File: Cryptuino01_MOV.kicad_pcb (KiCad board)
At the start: 2 copper layers, 37.9 x 31.2 mm, 31 parts, among them J1 USB_C_Receptacle_USB2.0, J2 Conn_01x06_Female, J3 Conn_01x08_Female, U1 FT245RL, U2 74HC02, U3 74HC00, U4 ATtiny4313-MU

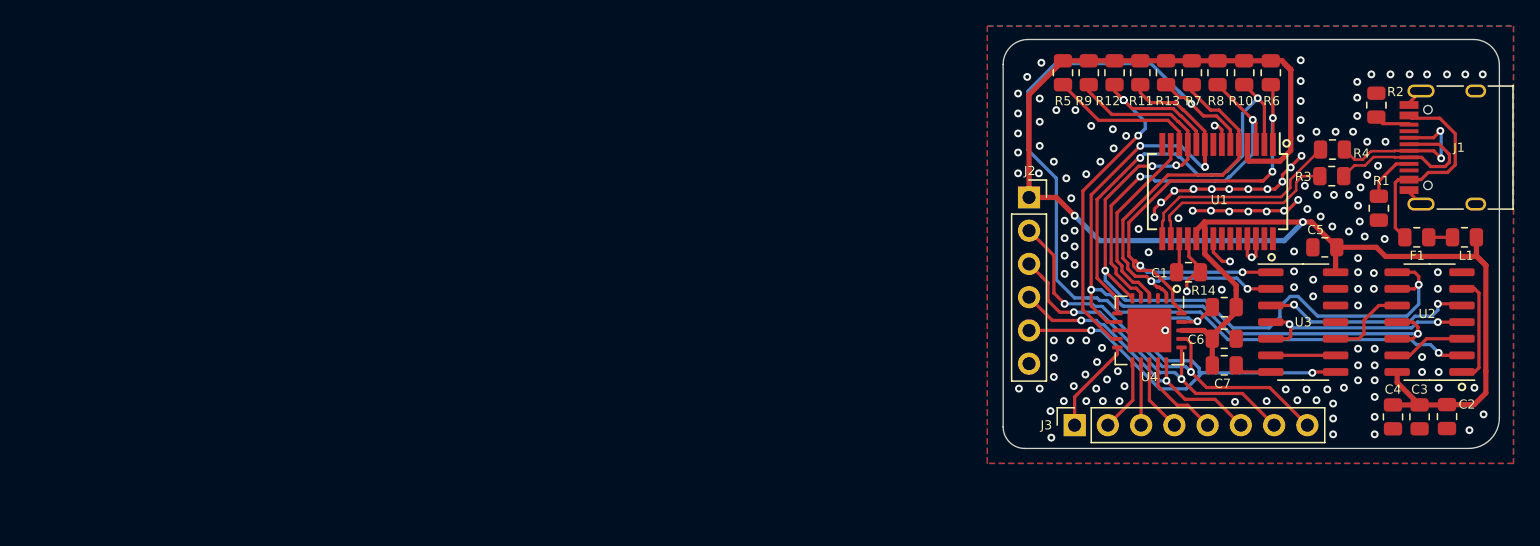
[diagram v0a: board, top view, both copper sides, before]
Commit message: done_nice_now
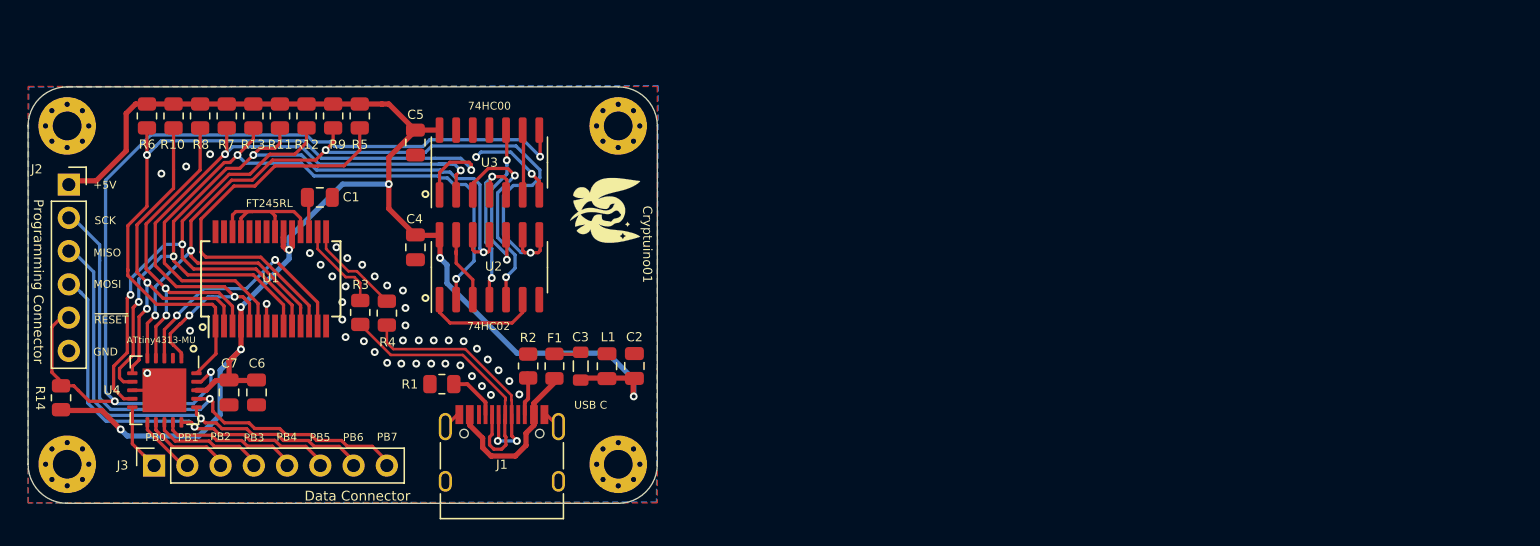
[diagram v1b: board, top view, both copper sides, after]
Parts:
- added G***: LOGO, FairyLogo:fairy_mask, F.Cu at (127.9, 67.2)
- added G***: LOGO, FairyLogo:fairy_silks, F.Cu at (128.0, 64.5)
- added REF**: KiCad-Logo2_6mm_SilkScreen, Symbol:KiCad-Logo2_6mm_SilkScreen, B.Cu at (103.6, 69.8)
- added REF**: MountingHole_2.2mm_M2_Pad_Via, MountingHole:MountingHole_2.2mm_M2_Pad_Via, F.Cu at (129.0, 58.0)
- added REF**: MountingHole_2.2mm_M2_Pad_Via, MountingHole:MountingHole_2.2mm_M2_Pad_Via, F.Cu at (86.9, 58.0)
- added REF**: MountingHole_2.2mm_M2_Pad_Via, MountingHole:MountingHole_2.2mm_M2_Pad_Via, F.Cu at (86.9, 83.9)
- added REF**: MountingHole_2.2mm_M2_Pad_Via, MountingHole:MountingHole_2.2mm_M2_Pad_Via, F.Cu at (129.0, 83.9)
- C1, C2, C3, C4, C5, C6, C7: footprint Resistor_SMD:R_0805_2012Metric -> Capacitor_SMD:C_0805_2012Metric
- F1: footprint Resistor_SMD:R_0805_2012Metric -> Fuse:Fuse_0805_2012Metric
- L1: footprint Resistor_SMD:R_0805_2012Metric -> Inductor_SMD:L_0805_2012Metric
- moved R14 89.1 mm to (86.4, 78.8), turned to 270 degrees
- moved R6 85.9 mm to (93.0, 57.3)
- moved R10 81.9 mm to (95.0, 57.3)
- moved R8 77.8 mm to (97.0, 57.3)
- moved J1 77.3 mm to (120.1, 84.1), turned to 0 degrees
- moved C7 76.1 mm to (99.2, 78.4), turned to 270 degrees
- moved C4 75.8 mm to (113.5, 67.3)
- moved U4 75.4 mm to (94.3, 78.2)
- moved R3 74.9 mm to (109.3, 72.3), turned to 270 degrees
- moved C6 74.0 mm to (101.3, 78.4), turned to 270 degrees
- moved R7 73.8 mm to (99.1, 57.3)
- moved J2 73.4 mm to (87.0, 62.5)
- moved R4 73.3 mm to (111.3, 72.3), turned to 270 degrees
- moved R1 72.8 mm to (115.5, 77.8), turned to 0 degrees
- moved U1 72.6 mm to (102.4, 69.7), turned to 90 degrees
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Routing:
- net ~RESET: track 40.7 -> 75.4 mm
- net /D7: track 72.3 -> 51.5 mm
- net Net-(R5-Pad2): track 11.3 -> 30.3 mm
- net /D1: track 36.1 -> 53.0 mm, vias 2 -> 4
- net GND: track 44.5 -> 27.7 mm, vias 153 -> 44
- net /D0: track 41.5 -> 56.6 mm, vias 4 -> 2
- net /D6: track 31.2 -> 43.1 mm, vias 3 -> 2
- net SCK: track 32.2 -> 42.0 mm, vias 2 -> 1
- net MOSI: track 21.7 -> 31.3 mm, vias 2 -> 1
- net USBD+: track 16.4 -> 7.61 mm
- net MISO: track 27.1 -> 35.7 mm, vias 2 -> 1
- net USBD-: track 14.9 -> 6.99 mm
- net /D-: track 13.1 -> 21.0 mm
- net /D3: track 62.0 -> 69.4 mm
- net Net-(U2-Pad10): track 6.35 -> 13.1 mm, vias 0 -> 2
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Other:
- board size 37.9 x 31.2 mm -> 48.1 x 31.8 mm
- net class My removed
- net class VBUS added: clearance 0.2, trace_width 0.3, via_dia 0.6, via_drill 0.3
- board text added: "+5V"
- board text added: "74HC00"
- board text added: "74HC02"
- board text added: "ATtiny4313-MU"
- board text added: "Cryptuino01"
- board text added: "Data Connector"
- board text added: "FT245RL"
- board text added: "GND"
- board text added: "MISO"
- board text added: "MOSI"
- board text added: "PB0"
- board text added: "PB1"
- board text added: "PB2"
- board text added: "PB3"
- board text added: "PB4"
- board text added: "PB5"
- board text added: "PB6"
- board text added: "PB7"
- board text added: "Programming Connector"
- board text added: "SCK"
- board text added: "USB C"
- board text added: "powered by Ksi0Na"
- board text added: "~RESET"
